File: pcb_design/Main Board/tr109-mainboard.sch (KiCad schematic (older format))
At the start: 24 parts, among them J1 Raspberry Pi Zero W, J2 ST7735_Screen, J3 Light_Board, J4 Cap_and_Bat, J5 Hall_1, J6 Conn_01x02_Female-Connector, J7 Hall_2, J8 Led_On, U1 CAP1208, U2 74HC595, U3 PAM8302AAS

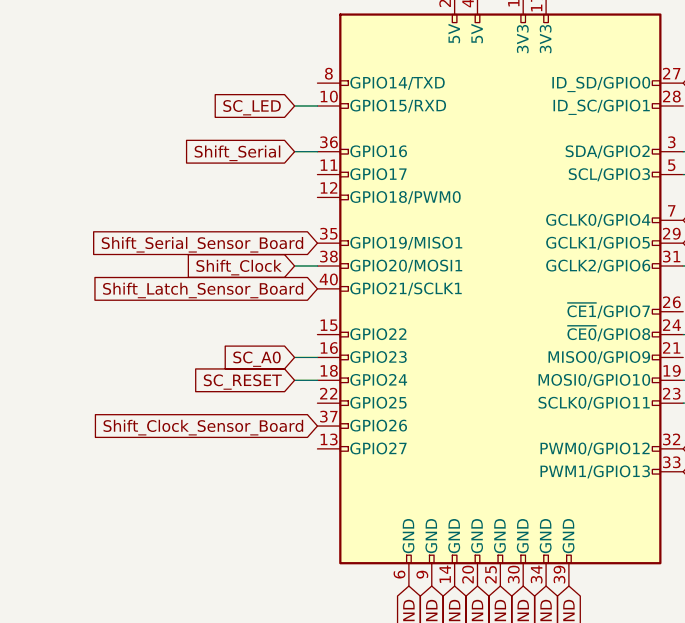
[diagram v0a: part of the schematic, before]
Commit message: Pcb and enclosure changes for proto 01
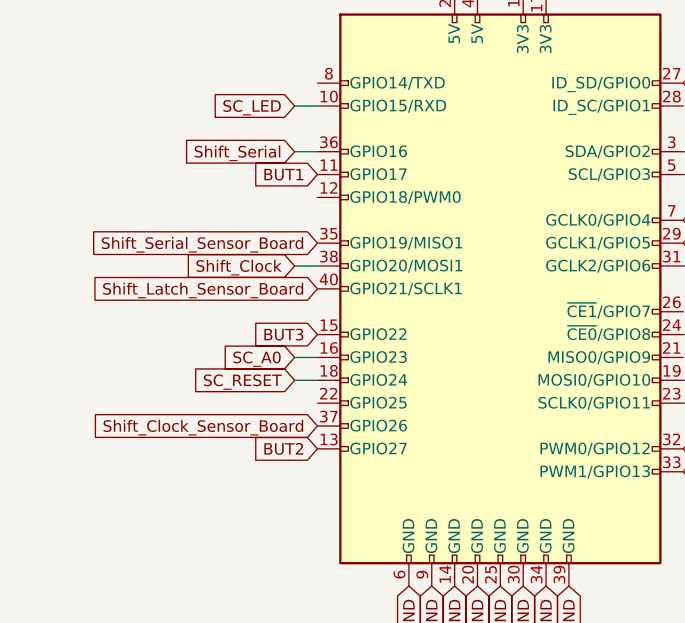
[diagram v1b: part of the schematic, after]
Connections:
- net labels added: BUT1, BUT2, BUT3
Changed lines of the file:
@@
 Text GLabel 9650 5000 0    50   Input ~ 0
 GND
+Text GLabel 1750 2050 0    50   Input ~ 0
+BUT1
+Text GLabel 1750 3250 0    50   Input ~ 0
+BUT2
+Text GLabel 1750 2750 0    50   Input ~ 0
+BUT3
 $EndSCHEMATC

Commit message: changes to shell and pcb
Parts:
- added J10: raw_audio_out, Connector_PinHeader_2.54mm:PinHeader_1x01_P2.54mm_Vertical, symbol Connector:Conn_01x01_Female
- added J9: i2c_bus, Connector_PinHeader_2.54mm:PinHeader_1x02_P2.54mm_Vertical, symbol Connector:Conn_01x02_Female
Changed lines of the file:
@@
 Text GLabel 1750 2750 0    50   Input ~ 0
 BUT3
+$Comp
+L Connector:Conn_01x02_Female J9
+U 1 1 610ACCCB
+P 9850 5600
+F 0 "J9" H 9878 5576 50  0000 L CNN
+F 1 "i2c_bus" H 9878 5485 50  0000 L CNN
+F 2 "Connector_PinHeader_2.54mm:PinHeader_1x02_P2.54mm_Vertical" H 9850 5600 50  0001 C CNN
+F 3 "~" H 9850 5600 50  0001 C CNN
+	1    9850 5600
+	1    0    0    -1
+$EndComp
+Text GLabel 9650 5700 0    50   Input ~ 0
+SDA
+Text GLabel 9650 5600 0    50   Input ~ 0
+SCL
+$Comp
+L Connector:Conn_01x01_Female J10
+U 1 1 610B2E38
+P 9850 6000
+F 0 "J10" H 9878 6026 50  0000 L CNN
+F 1 "raw_audio_out" H 9878 5935 50  0000 L CNN
+F 2 "Connector_PinHeader_2.54mm:PinHeader_1x01_P2.54mm_Vertical" H 9850 6000 50  0001 C CNN
+F 3 "~" H 9850 6000 50  0001 C CNN
+	1    9850 6000
+	1    0    0    -1
+$EndComp
+Text GLabel 9650 6000 0    50   Input ~ 0
+AUDIO
 $EndSCHEMATC
